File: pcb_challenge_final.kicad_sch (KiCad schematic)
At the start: 164 parts, among them J4 Conn_01x04_Pin, J5 Conn_01x04_Pin, Q15 Q_Dual_NPN_PNP_B1E2B2C2E1C1, Q16 Q_Dual_NPN_PNP_B1E2B2C2E1C1, Q17 Q_Dual_NPN_PNP_B1E2B2C2E1C1, Q18 Q_Dual_NPN_PNP_B1E2B2C2E1C1, Q19 Q_Dual_NPN_PNP_B1E2B2C2E1C1, Q20 Q_Dual_NPN_PNP_B1E2B2C2E1C1, Q21 Q_Dual_NPN_PNP_B1E2B2C2E1C1, Q22 Q_Dual_NPN_PNP_B1E2B2C2E1C1, Q23 Q_Dual_NPN_PNP_B1E2B2C2E1C1, Q24 Q_Dual_NPN_PNP_B1E2B2C2E1C1, Q25 Q_Dual_NPN_PNP_B1E2B2C2E1C1, Q26 Q_Dual_NPN_PNP_B1E2B2C2E1C1, Q27 Q_Dual_NPN_PNP_B1E2B2C2E1C1, Q28 Q_Dual_NPN_PNP_B1E2B2C2E1C1, Q29 Q_Dual_NPN_PNP_B1E2B2C2E1C1, SW1 SW_Push, SW2 SW_MEC_5G, SW3 SW_Push, U1 74AUP1G80, U10 NMUX1308BQ, U11 NMUX1308BQ, U12 NMUX1308BQ, U13 NMUX1308BQ, U14 NMUX1308BQ, U15 NMUX1308BQ, U16 NMUX1308BQ, U17 74AUP1G80, U18 74AHC1G86, U19 74AUP1G80, U20 74AUP1G80, U21 74LV1T08GV, U22 CD74HC283M96, U23 74LV1T08GV, U24 74LVC1GU04DRL, U25 ESP32-S3-MINI-1, U26 74LVC1GU04DRL, U27 74LV1T08GV, U28 CD74HC283M96, U29 NMUX1308BQ, U3 74AHC1G86, U30 NMUX1308BQ, U31 NMUX1308BQ, U32 NMUX1308BQ, U33 74AUP1G80, U34 74AUP1G80, U35 NMUX1308BQ, U36 NMUX1308BQ, U37 74AUP1G80, U38 74AUP1G80, U39 NMUX1308BQ, U4 74AUP1G80, U40 NMUX1308BQ, U41 NMUX1308BQ, U42 NMUX1308BQ, U43 NMUX1308BQ, U44 NMUX1308BQ, U45 74AUP1G80, U46 74AUP1G80, U47 74AUP1G80, U48 74AUP1G80, U49 74AUP1G80, U5 74AUP1G80, U50 74AUP1G80, U51 74LV1T08GV, U52 74AHC1G86, U53 74LVC1GU04DRL, U54 74LVC1GU04DRL, U55 74AHC1G86, U56 74AHC1G86, U57 74LVC1GU04DRL, U58 74LVC1GU04DRL, U59 74LV1T08GV, U6 74AUP1G80, U60 74AHC1G86, U61 74LVC1GU04DRL, U62 74LV1T08GV, U63 74LV1T08GV, U64 NMUX1308BQ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

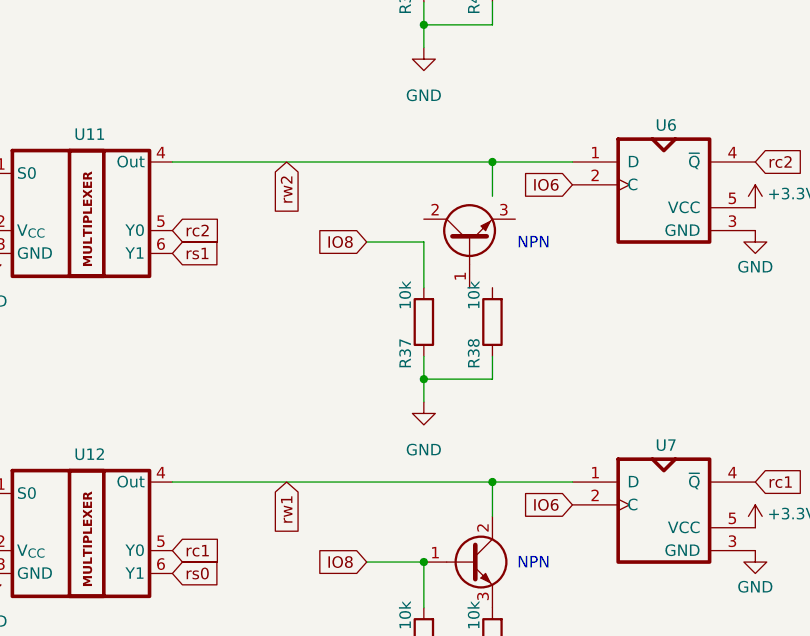
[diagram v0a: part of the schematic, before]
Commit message: Add files via upload
connected most of last things, still bunch of errors, running out of time
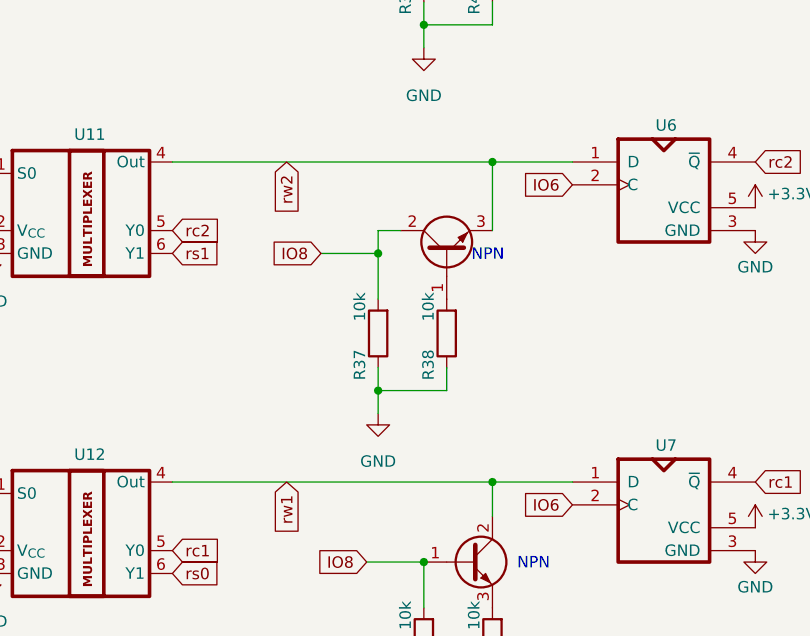
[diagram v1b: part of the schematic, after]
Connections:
- net IO8: now also Q19.2 (C1)
- net rw2: now also Q19.3 (E1)
- net at R38.2: now also Q19.1 (B1)
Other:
- moved on the sheet: R37, R38
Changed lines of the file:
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@@
 	(text "NPN\n"
 		(exclude_from_sim no)
-		(at 356.362 160.274 0)
+		(at 351.282 161.544 0)
 		(effects
 			(font
@@
 	)
 	(junction
+		(at 339.09 161.29)
+		(diameter 0)
+		(color 0 0 0 0)
+	)
+	(junction
 		(at 311.15 29.21)
 		(diameter 0)
@@
 	)
 	(junction
-		(at 344.17 175.26)
+		(at 339.09 176.53)
 		(diameter 0)
 		(color 0 0 0 0)
@@
 	(wire
 		(pts
+			(xy 339.09 158.75) (xy 339.09 161.29)
+		)
+		(stroke
+			(width 0)
+			(type default)
+		)
+	)
+	(wire
+		(pts
 			(xy 579.12 148.59) (xy 579.12 143.51)
 		)
@@
 	(wire
 		(pts
+			(xy 341.63 158.75) (xy 339.09 158.75)
+		)
+		(stroke
+			(width 0)
+			(type default)
+		)
+	)
+	(wire
+		(pts
 			(xy 585.47 21.59) (xy 585.47 25.4)
 		)
@@
 	(wire
 		(pts
-			(xy 337.82 160.02) (xy 344.17 160.02)
+			(xy 332.74 161.29) (xy 339.09 161.29)
 		)
 		(stroke
@@
 	(wire
 		(pts
-			(xy 351.79 151.13) (xy 351.79 154.94)
-		)
-		(stroke
-			(width 0)
-			(type default)
-		)
-	)
-	(wire
-		(pts
 			(xy 579.12 80.01) (xy 579.12 82.55)
 		)
@@
 	(wire
 		(pts
-			(xy 344.17 172.72) (xy 344.17 175.26)
+			(xy 339.09 173.99) (xy 339.09 176.53)
 		)
 		(stroke
@@
 	(wire
 		(pts
-			(xy 351.79 175.26) (xy 344.17 175.26)
+			(xy 346.71 176.53) (xy 339.09 176.53)
 		)
 		(stroke
@@
 	(wire
 		(pts
+			(xy 351.79 151.13) (xy 351.79 158.75)
+		)
+		(stroke
+			(width 0)
+			(type default)
+		)
+	)
+	(wire
+		(pts
 			(xy 36.83 74.93) (xy 35.56 74.93)
 		)
@@
 	(wire
 		(pts
-			(xy 351.79 172.72) (xy 351.79 175.26)
+			(xy 346.71 173.99) (xy 346.71 176.53)
 		)
 		(stroke
@@
 	(wire
 		(pts
-			(xy 344.17 165.1) (xy 344.17 160.02)
+			(xy 339.09 166.37) (xy 339.09 161.29)
 		)
 		(stroke
@@
 	(wire
 		(pts
-			(xy 344.17 177.8) (xy 344.17 175.26)
+			(xy 339.09 179.07) (xy 339.09 176.53)
 		)
 		(stroke
@@
 	(global_label "IO8"
 		(shape input)
-		(at 337.82 160.02 180)
+		(at 332.74 161.29 180)
 		(fields_autoplaced yes)
 		(effects
@@
 		)
 		(property "Intersheetrefs" "${INTERSHEET_REFS}"
-			(at 331.69 160.02 0)
+			(at 326.61 161.29 0)
 			(hide yes)
 			(show_name no)
@@
 	(symbol
 		(lib_id "power:GND")
-		(at 344.17 177.8 0)
+		(at 339.09 179.07 0)
 		(unit 1)
 		(body_style 1)
@@
 		(fields_autoplaced yes)
 		(property "Reference" "#PWR099"
-			(at 344.17 184.15 0)
+			(at 339.09 185.42 0)
 			(hide yes)
 			(show_name no)
@@
 		)
 		(property "Value" "GND"
-			(at 344.17 183.134 0)
+			(at 339.09 184.404 0)
 			(show_name no)
 			(do_not_autoplace no)
@@
 		)
 		(property "Footprint" ""
-			(at 344.17 177.8 0)
+			(at 339.09 179.07 0)
 			(hide yes)
 			(show_name no)
@@
 		)
 		(property "Datasheet" ""
-			(at 344.17 177.8 0)
+			(at 339.09 179.07 0)
 			(hide yes)
 			(show_name no)
@@
 		)
 		(property "Description" "Power symbol creates a global label with name \"GND\" , ground"
-			(at 344.17 177.8 0)
+			(at 339.09 179.07 0)
 			(hide yes)
 			(show_name no)
@@
 	(symbol
 		(lib_id "Device:R")
-		(at 344.17 168.91 180)
+		(at 339.09 170.18 180)
 		(unit 1)
 		(body_style 1)
@@
 		(dnp no)
 		(property "Reference" "R37"
-			(at 342.138 170.688 90)
+			(at 337.058 171.958 90)
 			(show_name no)
 			(do_not_autoplace no)
@@
 		)
 		(property "Value" "10k"
-			(at 342.138 164.338 90)
+			(at 337.058 165.608 90)
 			(show_name no)
 			(do_not_autoplace no)
@@
 		)
 		(property "Footprint" "Capacitor_SMD:C_0603_1608Metric"
-			(at 345.948 168.91 90)
+			(at 340.868 170.18 90)
 			(hide yes)
 			(show_name no)
@@
 		)
 		(property "Datasheet" "~"
-			(at 344.17 168.91 0)
+			(at 339.09 170.18 0)
 			(hide yes)
 			(show_name no)
@@
 		)
 		(property "Description" "Resistor"
-			(at 344.17 168.91 0)
+			(at 339.09 170.18 0)
 			(hide yes)
 			(show_name no)
@@
 	(symbol
 		(lib_id "Device:R")
-		(at 351.79 168.91 180)
+		(at 346.71 170.18 180)
 		(unit 1)
 		(body_style 1)
@@
 		(dnp no)
 		(property "Reference" "R38"
-			(at 349.758 170.688 90)
+			(at 344.678 171.958 90)
 			(show_name no)
 			(do_not_autoplace no)
@@
 		)
 		(property "Value" "10k"
-			(at 349.758 164.338 90)
+			(at 344.678 165.608 90)
 			(show_name no)
 			(do_not_autoplace no)
@@
 		)
 		(property "Footprint" "Capacitor_SMD:C_0603_1608Metric"
-			(at 353.568 168.91 90)
+			(at 348.488 170.18 90)
 			(hide yes)
 			(show_name no)
@@
 		)
 		(property "Datasheet" "~"
-			(at 351.79 168.91 0)
+			(at 346.71 170.18 0)
 			(hide yes)
 			(show_name no)
@@
 		)
 		(property "Description" "Resistor"
-			(at 351.79 168.91 0)
+			(at 346.71 170.18 0)
 			(hide yes)
 			(show_name no)
@@
 		(lib_name "Q_Dual_NPN_PNP_B1E2B2C2E1C1_1")
 		(lib_id "Transistor_BJT:Q_Dual_NPN_PNP_B1E2B2C2E1C1")
-		(at 349.25 160.02 90)
+		(at 346.71 161.29 90)
 		(unit 1)
 		(body_style 1)
@@
 		(fields_autoplaced yes)
 		(property "Reference" "Q19"
-			(at 347.9799 154.94 0)
+			(at 345.4399 156.21 0)
 			(hide yes)
 			(show_name no)
@@
 		)
 		(property "Value" "Q_Dual_NPN_PNP_B1E2B2C2E1C1"
-			(at 350.5199 154.94 0)
+			(at 347.9799 156.21 0)
 			(hide yes)
 			(show_name no)
@@
 		)
 		(property "Footprint" "Package_TO_SOT_SMD:SOT-1123"
-			(at 346.71 154.94 0)
+			(at 344.17 156.21 0)
 			(hide yes)
 			(show_name no)
@@
 		)
 		(property "Datasheet" ""
-			(at 349.25 160.02 0)
+			(at 346.71 161.29 0)
 			(hide yes)
 			(show_name no)
@@
 		)
 		(property "Description" "Dual NPN/PNP transistor, 6 pin package"
-			(at 349.25 160.02 0)
+			(at 346.71 161.29 0)
 			(hide yes)
 			(show_name no)
